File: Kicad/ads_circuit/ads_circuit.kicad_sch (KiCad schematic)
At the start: 9 parts, among them J1 Con

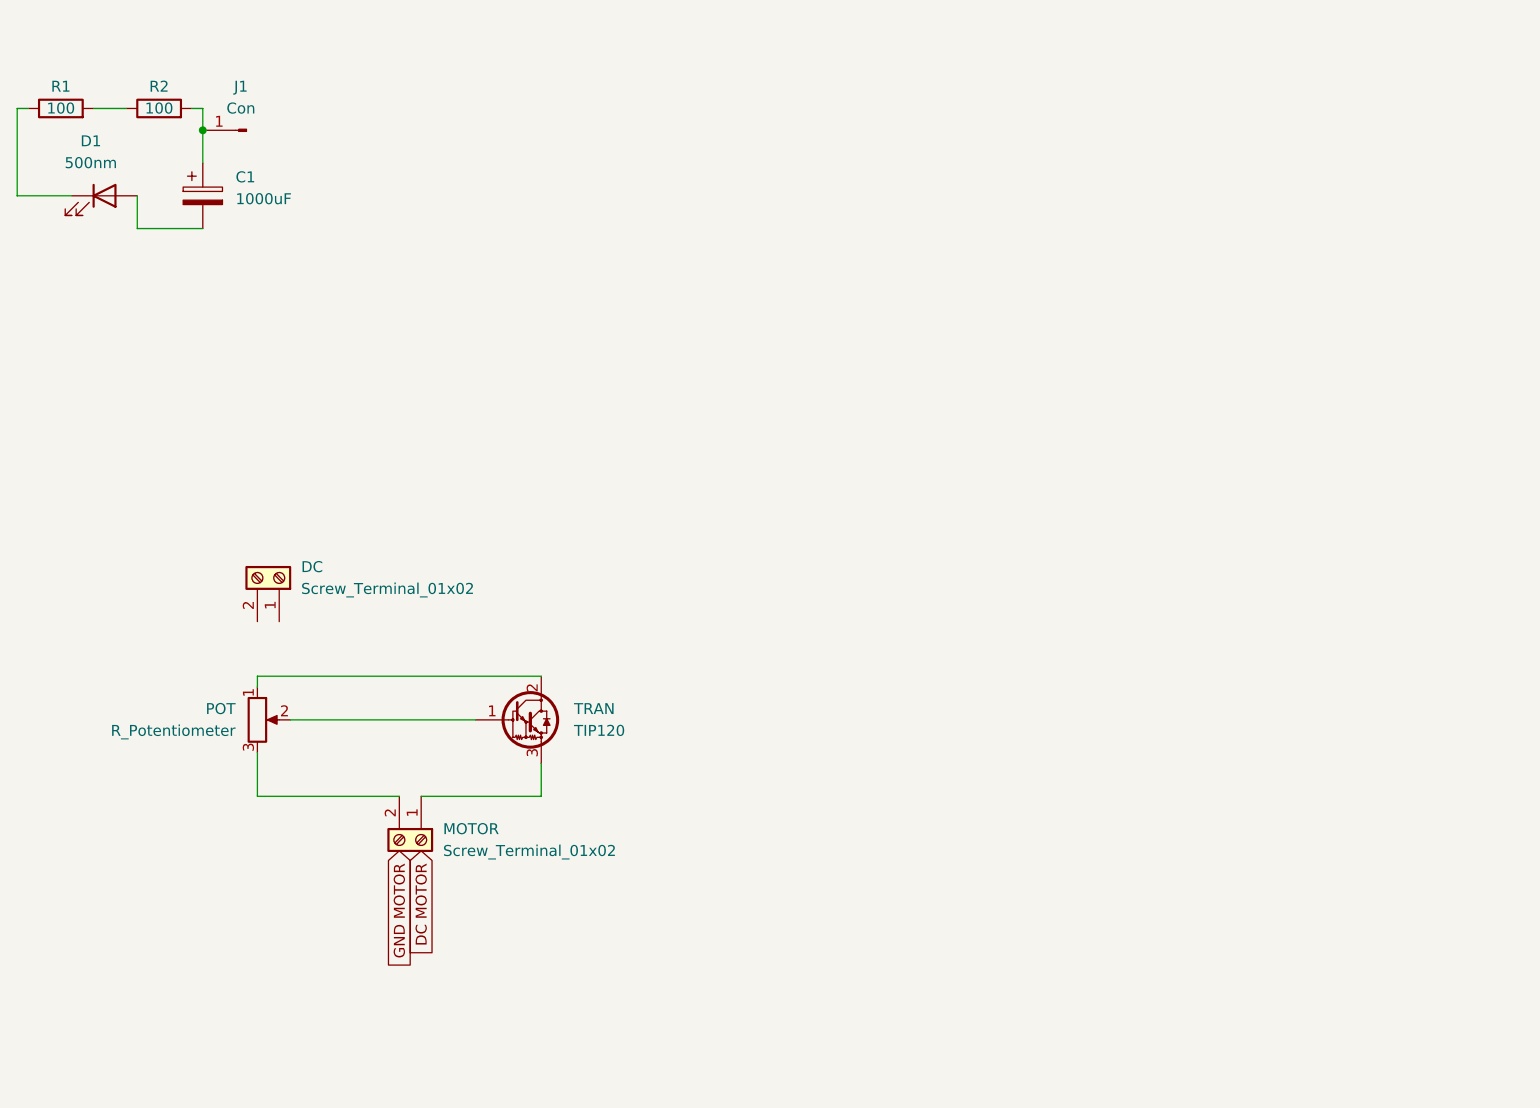
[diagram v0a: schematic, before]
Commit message: Kicad scheme
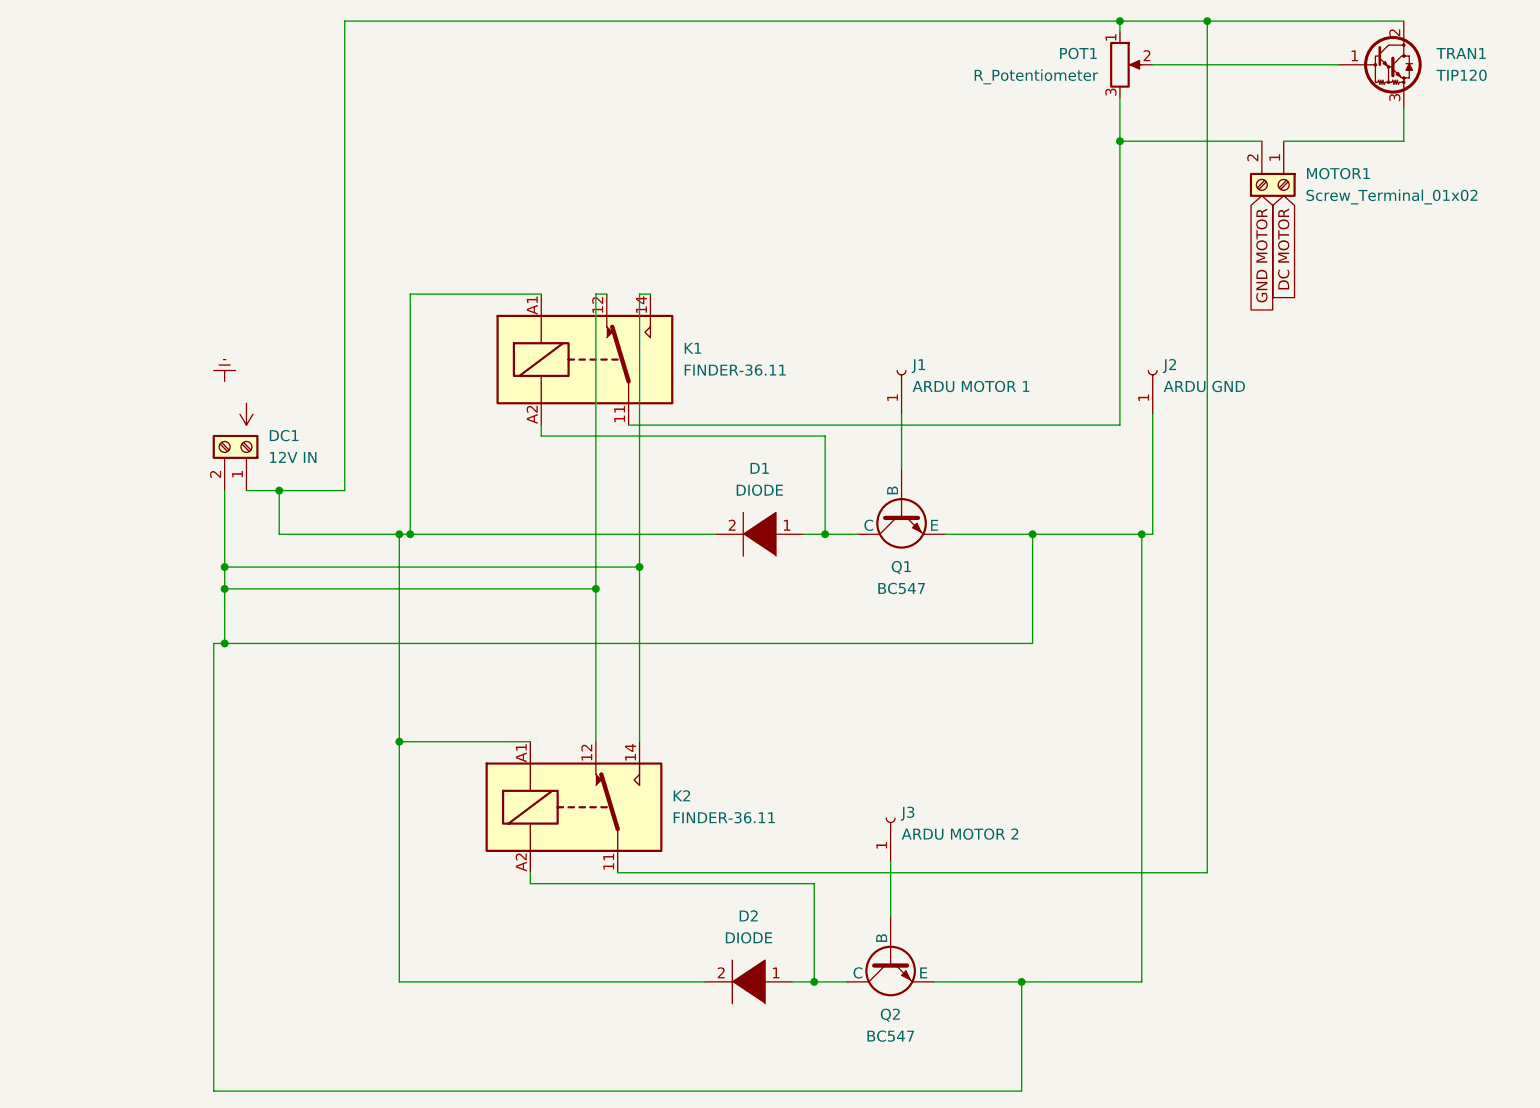
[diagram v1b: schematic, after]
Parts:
- removed C1: 1000uF, Capacitor_THT:CP_Radial_D10.0mm_P5.00mm, symbol Device:C_Polarized
- removed D1: 500nm, LED_THT:LED_D5.0mm, symbol Device:LED
- removed J1: Con, Connector_PinHeader_2.54mm:PinHeader_1x01_P2.54mm_Vertical, symbol Connector:Conn_01x01_Male
- removed R1, R2: 100, Resistor_THT:R_Axial_DIN0204_L3.6mm_D1.6mm_P7.62mm_Horizontal, symbol Device:R
- added D1, D2: DIODE, Diode_THT:D_A-405_P7.62mm_Horizontal, symbol pspice:DIODE
- added J1: ARDU MOTOR 1, Connector_PinHeader_1.00mm:PinHeader_1x01_P1.00mm_Vertical, symbol Connector:Conn_01x01_Female
- added J2: ARDU GND, Connector_PinHeader_1.00mm:PinHeader_1x01_P1.00mm_Vertical, symbol Connector:Conn_01x01_Female
- added J3: ARDU MOTOR 2, Connector_PinHeader_1.00mm:PinHeader_1x01_P1.00mm_Vertical, symbol Connector:Conn_01x01_Female
- added K1, K2: FINDER-36.11, Relay_THT:Relay_SPDT_Finder_36.11, symbol Relay:FINDER-36.11
- added Q1, Q2: BC547, Package_TO_SOT_THT:TO-92_Inline, symbol Transistor_BJT:BC547
- DC1: renamed from DC; value Screw_Terminal_01x02 -> 12V IN; footprint (none) -> TerminalBlock_RND:TerminalBlock_RND_205-00001_1x02_P5.00mm_Horizontal
- MOTOR1: renamed from MOTOR; footprint (none) -> TerminalBlock_RND:TerminalBlock_RND_205-00001_1x02_P5.00mm_Horizontal
- renumbered POT to POT1, TRAN to TRAN1
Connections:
- net at POT1.1, TRAN1.2 (C): now also DC1.1 (Pin_1), D1.2 (A), D2.2 (A), K1.A1, K2.11, K2.A1
- net at MOTOR1.2 (Pin_2), POT1.3: now also K1.11
- net at DC1.2 (Pin_2): now also J2.1 (Pin_1), K1.12, K1.14, K2.12, K2.14, Q1.3 (E), Q2.3 (E)
- new net: J3.1 (Pin_1), Q2.2 (B)
- new net: D2.1 (K), K2.A2, Q2.1 (C)
- new net: D1.1 (K), K1.A2, Q1.1 (C)
- new net: J1.1 (Pin_1), Q1.2 (B)
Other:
- moved on the sheet: DC1, MOTOR1, POT1, TRAN1
